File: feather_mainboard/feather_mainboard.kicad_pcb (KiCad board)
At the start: 2 copper layers, 60 x 60 mm, 0 parts

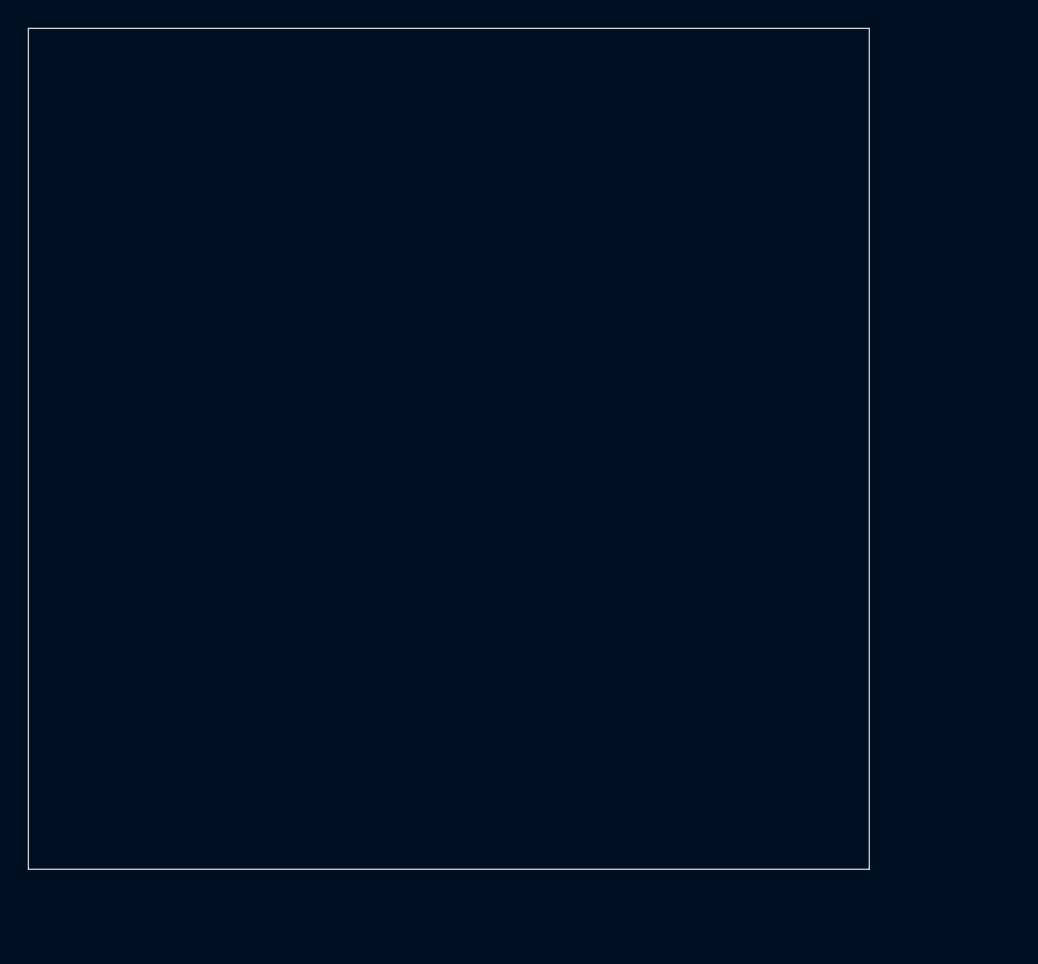
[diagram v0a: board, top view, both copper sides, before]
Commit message: finished mainboard design, need to do the routing
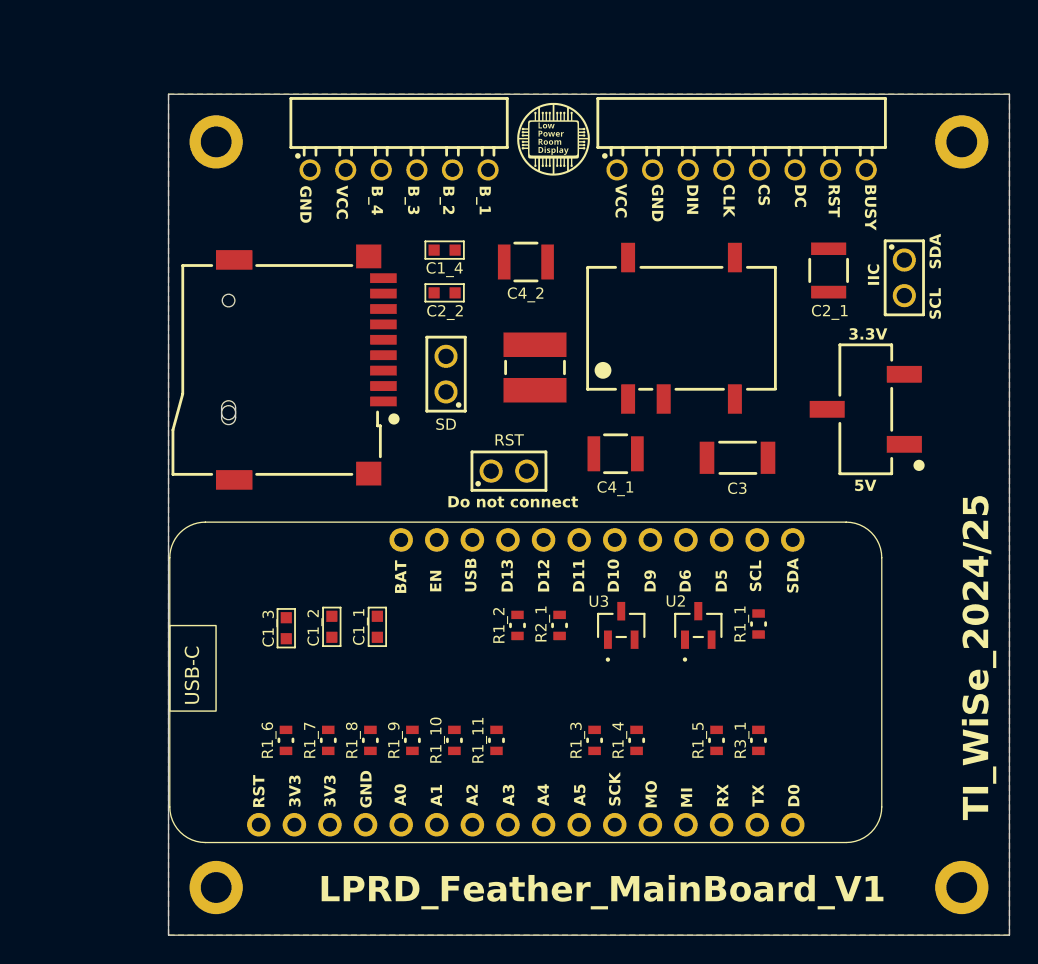
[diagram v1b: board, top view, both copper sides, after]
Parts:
- added C1_1: 100nF, Custom footprints:WCAP-CSGP_0603_R, F.Cu at (134.9, 107.7)
- added C1_2: 100nF, Custom footprints:WCAP-CSGP_0603_R, F.Cu at (131.7, 107.7)
- added C1_3: 100nF, Custom footprints:WCAP-CSGP_0603_R, F.Cu at (128.4, 107.8)
- added C1_4: 100nF, Custom footprints:WCAP-CSGP_0603_R, F.Cu at (139.7, 80.8)
- added C2_1: 10µF, Custom footprints:WCAP-CSGP_1210_H2.0, F.Cu at (167.1, 82.3)
- added C2_2: 10µF, Custom footprints:WCAP-CSGP_0603_R, F.Cu at (139.7, 83.9)
- added C3: 470pF, Custom footprints:WCAP-CSMH_1808_H2.0, F.Cu at (160.6, 95.6)
- added C4_1: 4.7µF, Custom footprints:WCAP-CSGP_1210_H2.0, F.Cu at (151.9, 95.3)
- added C4_2: 4.7µF, Custom footprints:WCAP-CSGP_1210_H2.0, F.Cu at (145.5, 81.7)
- added G***: LOGO, Custom footprints:Logo, F.Cu at (147.5, 72.9)
- added G***: LOGO, Custom footprints:Logo, B.Cu at (147.4, 72.9)
- added H1: MountingHole_Pad, MountingHole:MountingHole_2.2mm_M2_DIN965_Pad, F.Cu at (176.6, 73.1)
- added H2: MountingHole_Pad, MountingHole:MountingHole_2.2mm_M2_DIN965_Pad, F.Cu at (123.4, 73.1)
- added H3: MountingHole_Pad, MountingHole:MountingHole_2.2mm_M2_DIN965_Pad, F.Cu at (176.6, 126.3)
- added H4: MountingHole_Pad, MountingHole:MountingHole_2.2mm_M2_DIN965_Pad, F.Cu at (123.4, 126.3)
- added IIC: 61300211121, Custom footprints:61300211121, F.Cu at (172.5, 82.8)
- added J1: 61900819521, Custom footprints:61900819521, F.Cu at (160.9, 71.8)
- added J2: 61900619521, Custom footprints:61900619521, F.Cu at (136.4, 71.8)
- added J4: 693071020811, Custom footprints:693071020811, F.Cu at (124.3, 89.4)
- added L1: 6.8µH, Custom footprints:WE-PD2_4532, F.Cu at (146.2, 89.2)
- added R1_1: 10kΩ, Custom footprints:WRIS-RSKS_0603_REFLOW, F.Cu at (162.1, 107.5)
- added R1_10: 10kΩ, Custom footprints:WRIS-RSKS_0603_REFLOW, F.Cu at (140.4, 115.8)
- added R1_11: 10kΩ, Custom footprints:WRIS-RSKS_0603_REFLOW, F.Cu at (143.4, 115.8)
- added R1_2: 10kΩ, Custom footprints:WRIS-RSKS_0603_REFLOW, F.Cu at (144.9, 107.6)
- added R1_3: 10kΩ, Custom footprints:WRIS-RSKS_0603_REFLOW, F.Cu at (150.4, 115.8)
- added R1_4: 10kΩ, Custom footprints:WRIS-RSKS_0603_REFLOW, F.Cu at (153.4, 115.8)
- added R1_5: 10kΩ, Custom footprints:WRIS-RSKS_0603_REFLOW, F.Cu at (159.1, 115.8)
- added R1_6: 10kΩ, Custom footprints:WRIS-RSKS_0603_REFLOW, F.Cu at (128.4, 115.8)
- added R1_7: 10kΩ, Custom footprints:WRIS-RSKS_0603_REFLOW, F.Cu at (131.4, 115.8)
- added R1_8: 10kΩ, Custom footprints:WRIS-RSKS_0603_REFLOW, F.Cu at (134.4, 115.8)
- added R1_9: 10kΩ, Custom footprints:WRIS-RSKS_0603_REFLOW, F.Cu at (137.4, 115.8)
- added R2_1: 180Ω, Custom footprints:WRIS-RSKS_0603_REFLOW, F.Cu at (147.9, 107.6)
- added R3_1: 75kΩ, Custom footprints:WRIS-RSKS_0603_REFLOW, F.Cu at (162.1, 115.8)
- added RST: 61300211121, Custom footprints:61300211121, F.Cu at (144.3, 96.6)
- added S1: 450406020024, Custom footprints:450406020024, F.Cu at (169.8, 92.2)
- added SD: 61300211121, Custom footprints:61300211121, F.Cu at (139.8, 89.7)
- added U1: Adafruit ESP32-S3 Feather, Custom footprints:Adafruit ESP32-S3 Feather 4MB Flash 2MB PSRAM, F.Cu at (144.4, 95.7)
- added U2: SI2307CDS-T1-BE3, Custom footprints:SOT-23_VIS, F.Cu at (157.8, 107.6)
- added U3: 2N7002K-T1-GE3, Custom footprints:SOT_02K-T1-GE3_VIS, F.Cu at (152.3, 107.6)
- added U4: WPME-FISM_SMT-8, Custom footprints:WPME-FISM_SMT-8_L13.2W11.4H7.25, F.Cu at (156.6, 86.4)
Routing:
- added copper zone on B.Cu, net GND
- added copper zone on F.Cu, net GND
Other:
- board text added: "3.3V"
- board text added: "5V"
- board text added: "BUSY"
- board text added: "B_1"
- board text added: "B_2"
- board text added: "B_3"
- board text added: "B_4"
- board text added: "CLK"
- board text added: "CS"
- board text added: "DC"
- board text added: "DIN"
- board text added: "Do not connect"
- board text added: "GND"
- board text added: "IIC"
- board text added: "LPRD_Feather_MainBoard_V1"
- board text added: "RST"
- board text added: "SCL"
- board text added: "SDA"
- board text added: "TI_WiSe_2024/25"
- board text added: "VCC"
